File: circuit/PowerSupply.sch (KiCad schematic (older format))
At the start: 16 parts, among them CN1 Battery, CN2 Battery, Q1 IRLML6402, SW1 SW_SPDT, U1 NJM7805S, U4 ADP7182AUJZ-3.3

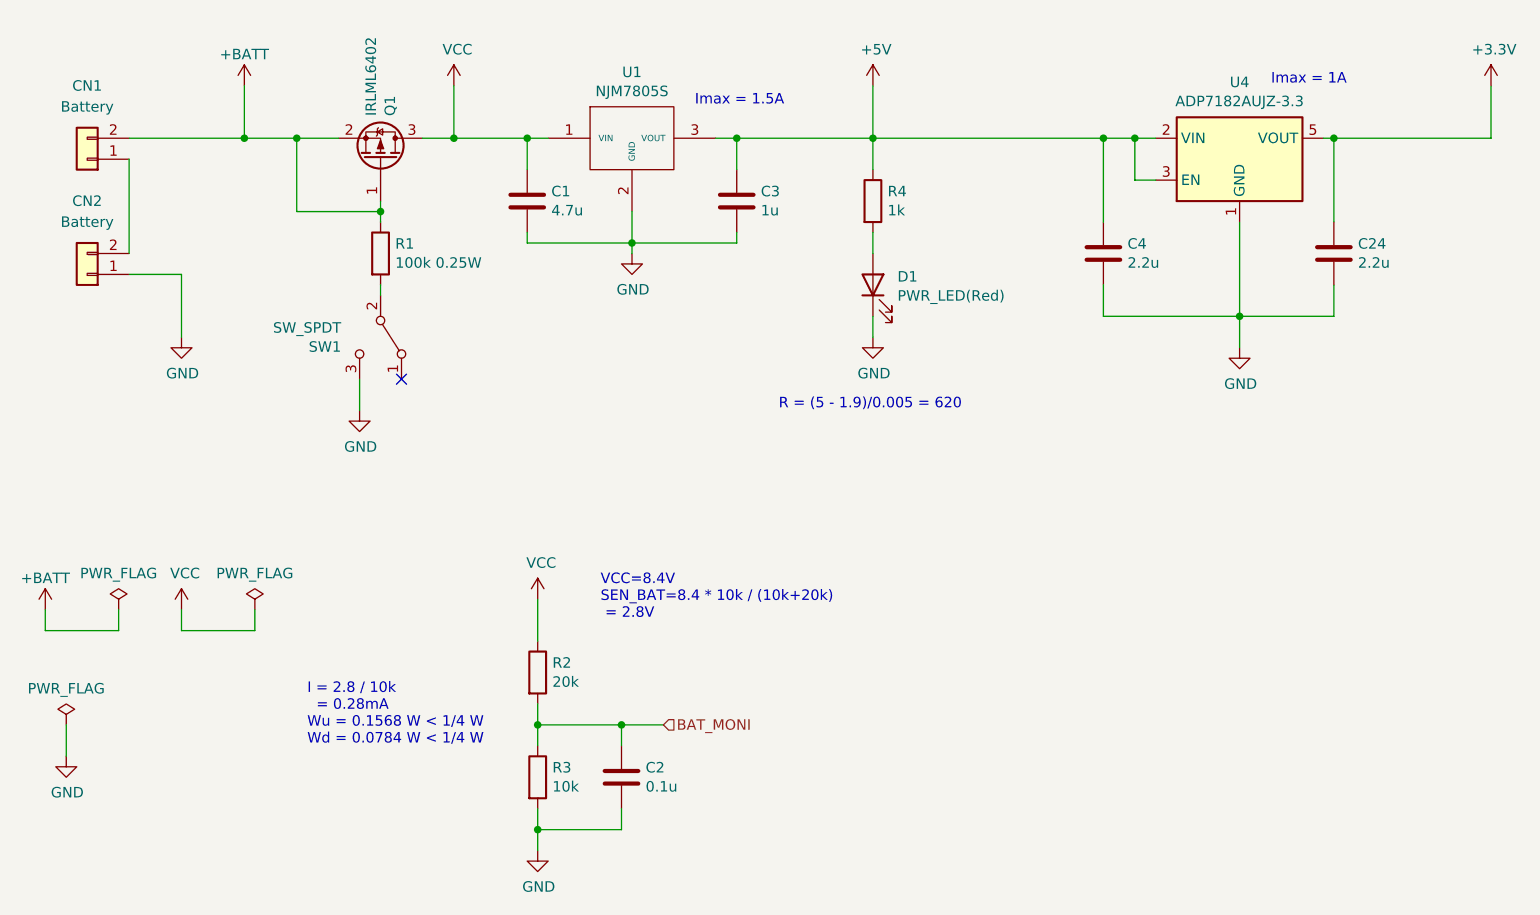
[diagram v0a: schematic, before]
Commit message: ヨー角ヨー角ヨー角
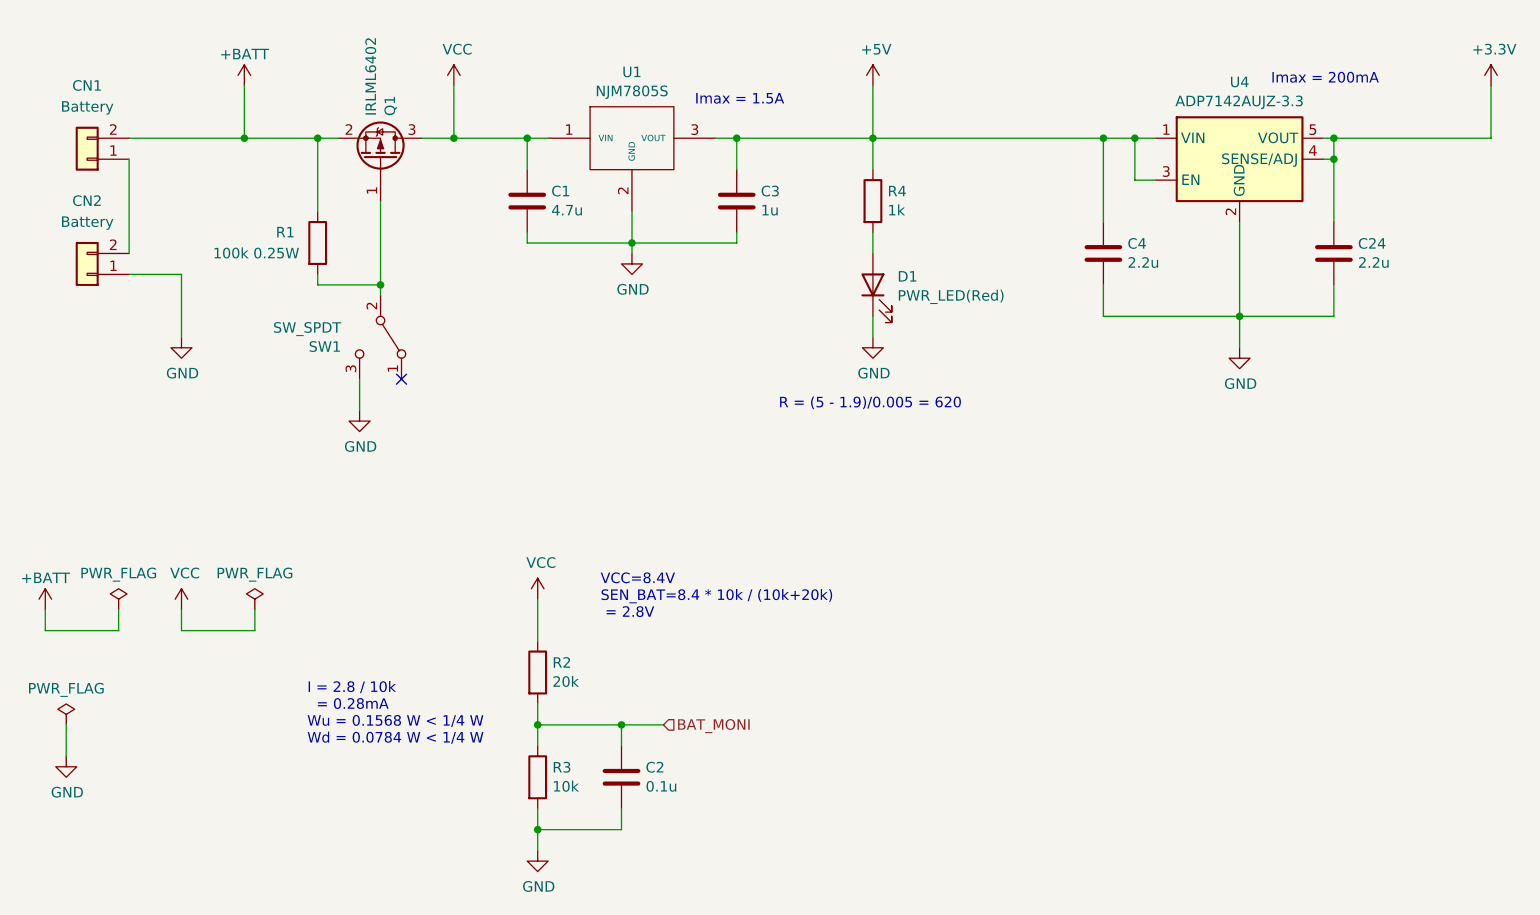
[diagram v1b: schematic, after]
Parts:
- removed U4: ADP7182AUJZ-3.3, Package_TO_SOT_SMD:TSOT-23-5, symbol Regulator_Linear:ADP7182AUJZ-3.3
- added U4: ADP7142AUJZ-3.3, Package_TO_SOT_SMD:TSOT-23-5, symbol Regulator_Linear:ADP7142AUJZ-3.3
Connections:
- net +3V3: now also U4.4 (SENSE/ADJ), U4.5 (VOUT)
- net +5V: now also U4.1 (VIN), U4.3 (EN)
- net +BATT: no longer Q1.1 (G)
- net GND: now also U4.2 (GND)
- net at R1.2, SW1.2 (B): now also Q1.1 (G)
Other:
- note added: "Imax = 200mA"
- note removed: "Imax = 1A"
- moved on the sheet: R1
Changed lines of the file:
@@
 L Device:R R1
 U 1 1 5F95E89C
-P 2400 1800
-F 0 "R1" H 2470 1846 50  0000 L CNN
-F 1 "100k 0.25W" H 2470 1755 50  0000 L CNN
-F 2 "Resistor_SMD:R_0603_1608Metric" V 2330 1800 50  0001 C CNN
-F 3 "" H 2400 1800 50  0001 C CNN
-	1    2400 1800
+P 2100 1750
+F 0 "R1" H 1900 1800 50  0000 L CNN
+F 1 "100k 0.25W" H 1600 1700 50  0000 L CNN
+F 2 "Resistor_SMD:R_0603_1608Metric" V 2030 1750 50  0001 C CNN
+F 3 "" H 2100 1750 50  0001 C CNN
+	1    2100 1750
 	1    0    0    -1
 $EndComp
@@
 Wire Wire Line
 	1450 1900 1450 2200
-Wire Wire Line
-	2400 1550 2400 1600
-Connection ~ 2400 1600
 $Comp
 L Switch:SW_SPDT SW1
@@
 Wire Wire Line
 	2300 2400 2300 2550
-Wire Wire Line
-	2400 2000 2400 1950
 $Comp
 L Device:LED D1
@@
 Connection ~ 4100 1250
 Wire Wire Line
-	1750 1250 2000 1250
-Wire Wire Line
-	2400 1600 2000 1600
-Wire Wire Line
-	2000 1600 2000 1250
-Wire Wire Line
-	2400 1600 2400 1650
-Connection ~ 2000 1250
-Wire Wire Line
-	2000 1250 2200 1250
-Wire Wire Line
 	2600 1250 2750 1250
 Connection ~ 2750 1250
@@
 	5850 1950 5850 2100
 Wire Wire Line
-	6950 1250 6950 1650
+	6950 1250 6950 1350
 Wire Wire Line
 	7700 1000 7700 1250
@@
 Imax = 1.5A\n
 Text Notes 6650 1000 0    50   ~ 0
-Imax = 1A
+Imax = 200mA
 Wire Wire Line
 	6500 2100 6500 2250
@@
 Wire Wire Line
 	6500 2100 6950 2100
-$Comp
-L Regulator_Linear:ADP7182AUJZ-3.3 U4
-U 1 1 5FB8CF9C
-P 6500 1350
-F 0 "U4" H 6500 983 50  0000 C CNN
-F 1 "ADP7182AUJZ-3.3" H 6500 1074 50  0000 C CNN
-F 2 "Package_TO_SOT_SMD:TSOT-23-5" H 6500 950 50  0001 C CIN
-F 3 "https://www.analog.com/media/en/technical-documentation/data-sheets/ADP7182.pdf" H 6500 850 50  0001 C CNN
-	1    6500 1350
-	1    0    0    1
-$EndComp
 Wire Wire Line
 	5850 1250 6000 1250
@@
 Wire Wire Line
 	6950 1950 6950 2100
+Wire Wire Line
+	2400 1550 2400 1950
+$Comp
+L Regulator_Linear:ADP7142AUJZ-3.3 U4
+U 1 1 600DD8DD
+P 6500 1350
+F 0 "U4" H 6500 1717 50  0000 C CNN
+F 1 "ADP7142AUJZ-3.3" H 6500 1626 50  0000 C CNN
+F 2 "Package_TO_SOT_SMD:TSOT-23-5" H 6500 950 50  0001 C CIN
+F 3 "https://www.analog.com/media/en/technical-documentation/data-sheets/ADP7142.pdf" H 6500 850 50  0001 C CNN
+	1    6500 1350
+	1    0    0    -1
+$EndComp
+Wire Wire Line
+	6900 1350 6950 1350
+Connection ~ 6950 1350
+Wire Wire Line
+	6950 1350 6950 1650
+Wire Wire Line
+	2100 1600 2100 1250
+Wire Wire Line
+	1750 1250 2100 1250
+Connection ~ 2100 1250
+Wire Wire Line
+	2100 1250 2200 1250
+Wire Wire Line
+	2100 1900 2100 1950
+Wire Wire Line
+	2100 1950 2400 1950
+Connection ~ 2400 1950
+Wire Wire Line
+	2400 1950 2400 2000
 $EndSCHEMATC
